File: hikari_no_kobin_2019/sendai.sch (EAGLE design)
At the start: 4 parts

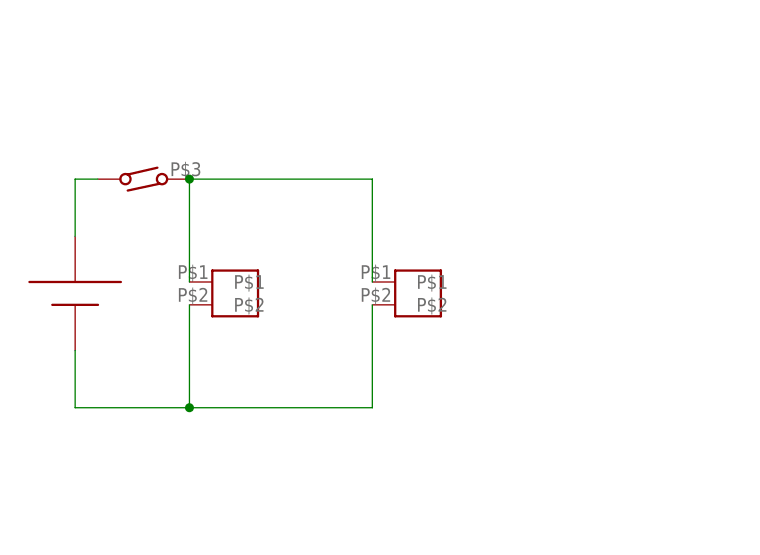
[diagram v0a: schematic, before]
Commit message: 20190905
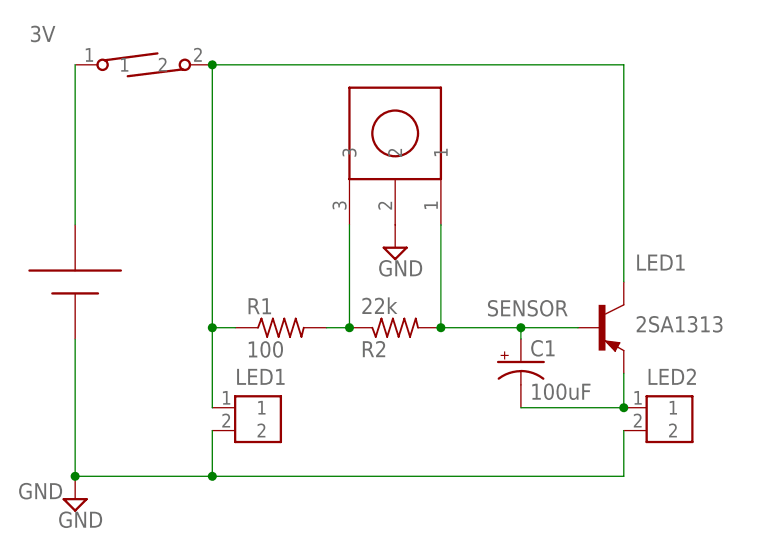
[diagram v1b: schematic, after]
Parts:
- added C1: 100uF, MATHRAX-a:CPOL-USTT2D6
- added R1: 100, MATHRAX-a:R-US_R0603
- added R2: 22k, MATHRAX-a:R-US_R0603
- added T1: 2SA1313, DC_LOAD_AU:-PNP-SOT23-BEC
- added U$5: OSRB38C9AA, sendai:OSRB38C9AA
- U$1: value CR2032_CR2032 -> CR2032_VCR2032_V; device sendai:CR2032_CR2032 -> sendai:CR2032_VCR2032_V
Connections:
- removed net N$1: U$2.P$1, U$3.P$1, U$4.P$1
- removed net N$2: U$1.-, U$2.P$2, U$3.P$2
- removed net N$3: U$1.+, U$4.P$2
- new net 3V: U$1.+, U$4.1
- new net GND: U$1.-, U$2.2, U$3.2, U$5.2
- new net LED1: R1.1, T1.C, U$2.1, U$4.2
- new net LED2: C1.-, T1.E, U$3.1
- new net SENSOR: C1.+, R2.2, T1.B, U$5.1
- new net V: R1.2, R2.1, U$5.3
